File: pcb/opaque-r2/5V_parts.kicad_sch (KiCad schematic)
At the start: 14 parts

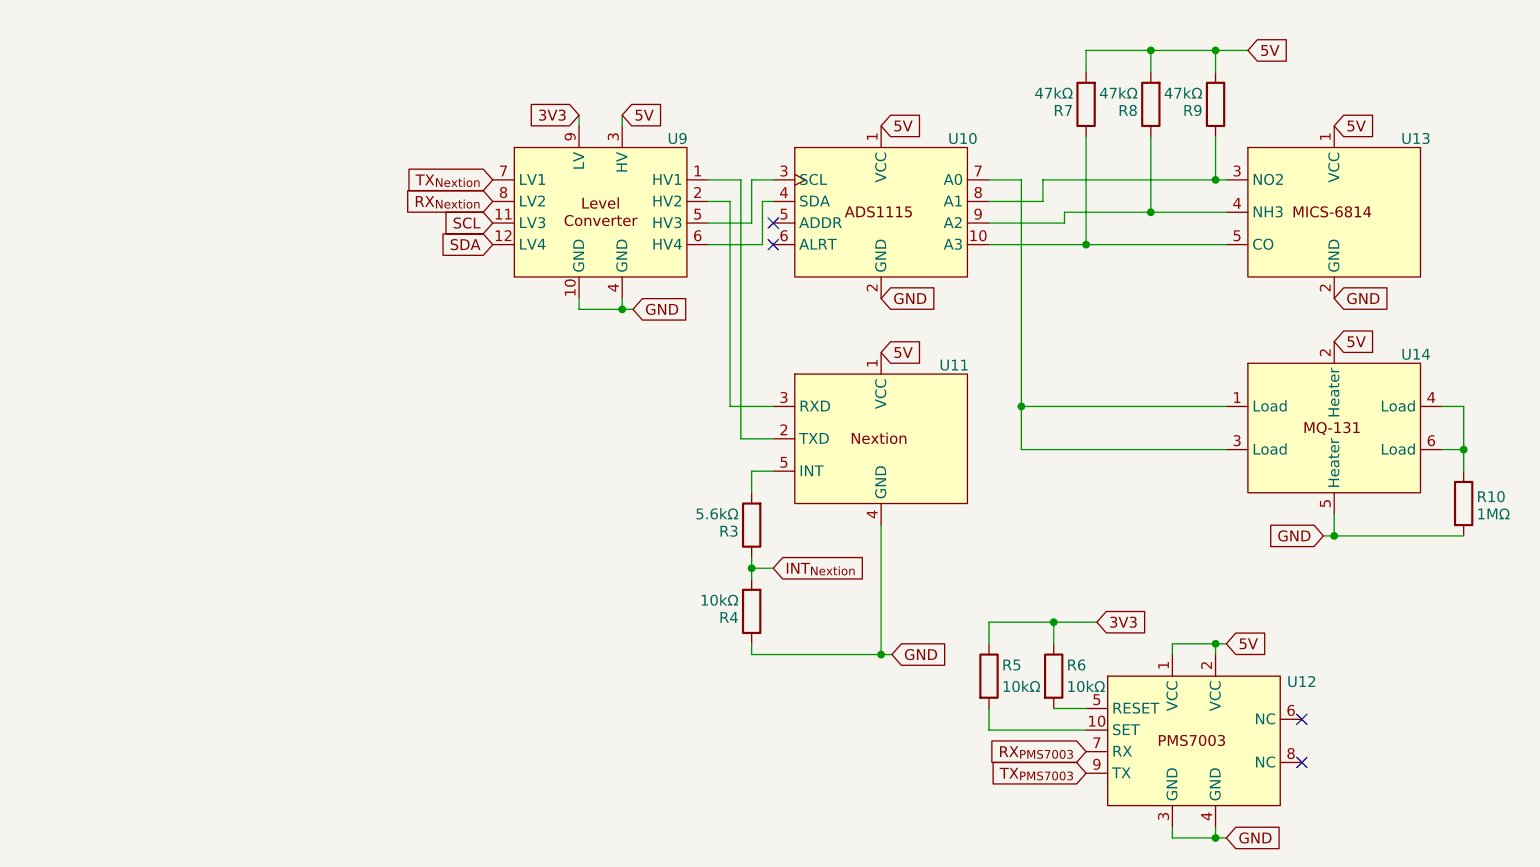
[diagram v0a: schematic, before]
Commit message: Writtin code
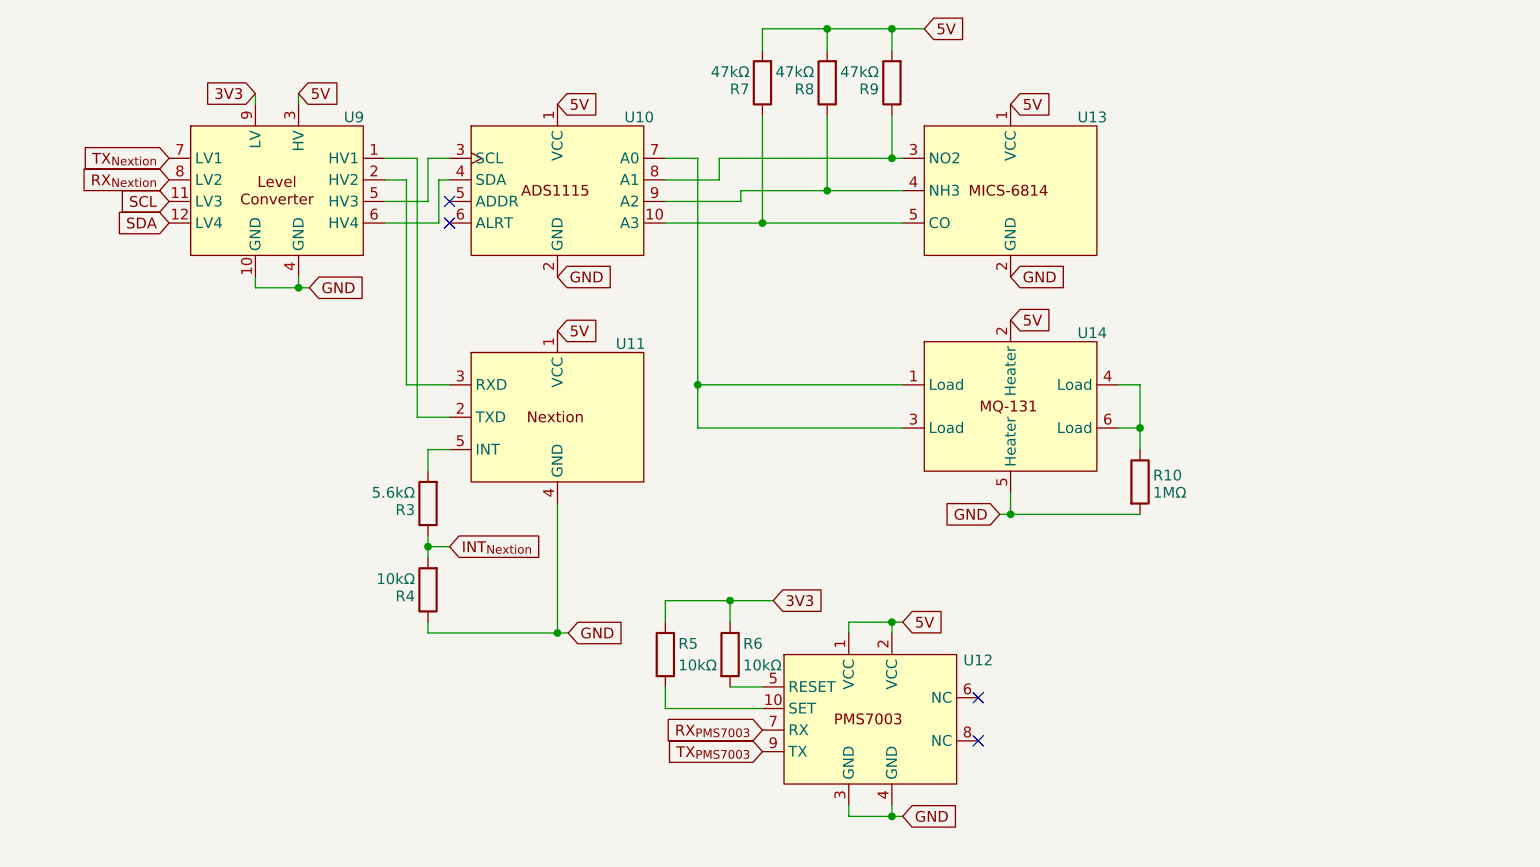
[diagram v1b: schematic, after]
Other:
- company: Barkın Özsoy (barkolorious) -> (none)
- title: opaque: Open-source Portable Air QUality Equipment -> Açık-kaynaklı Taşınabilir Hava Kalitesi Ölçüm Kitleri
- moved on the sheet: R10, R3, R4, R5, R6, R7, R8, R9, U10, U11, U12, U13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
